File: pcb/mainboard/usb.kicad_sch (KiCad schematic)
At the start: 39 parts

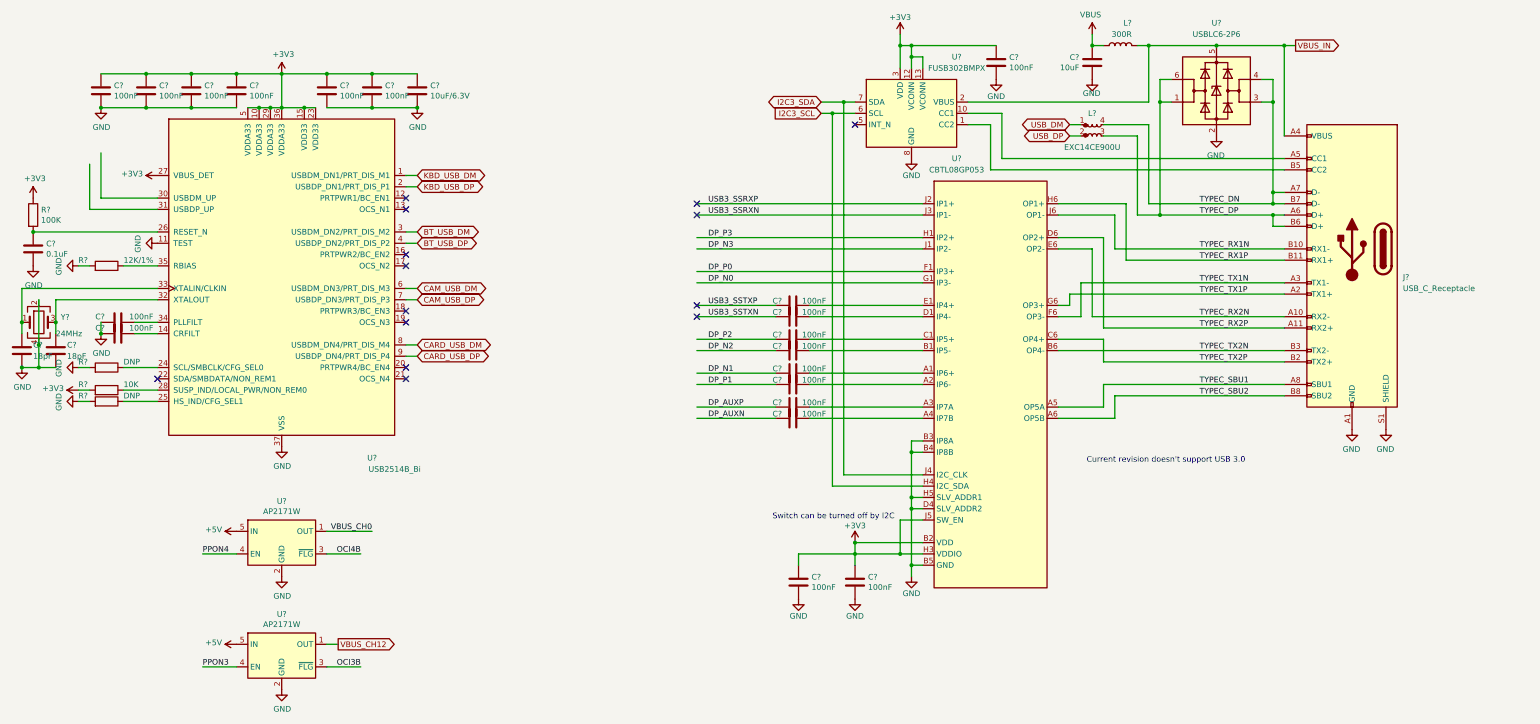
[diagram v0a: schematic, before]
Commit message: - pcb: working on r0p1 sch
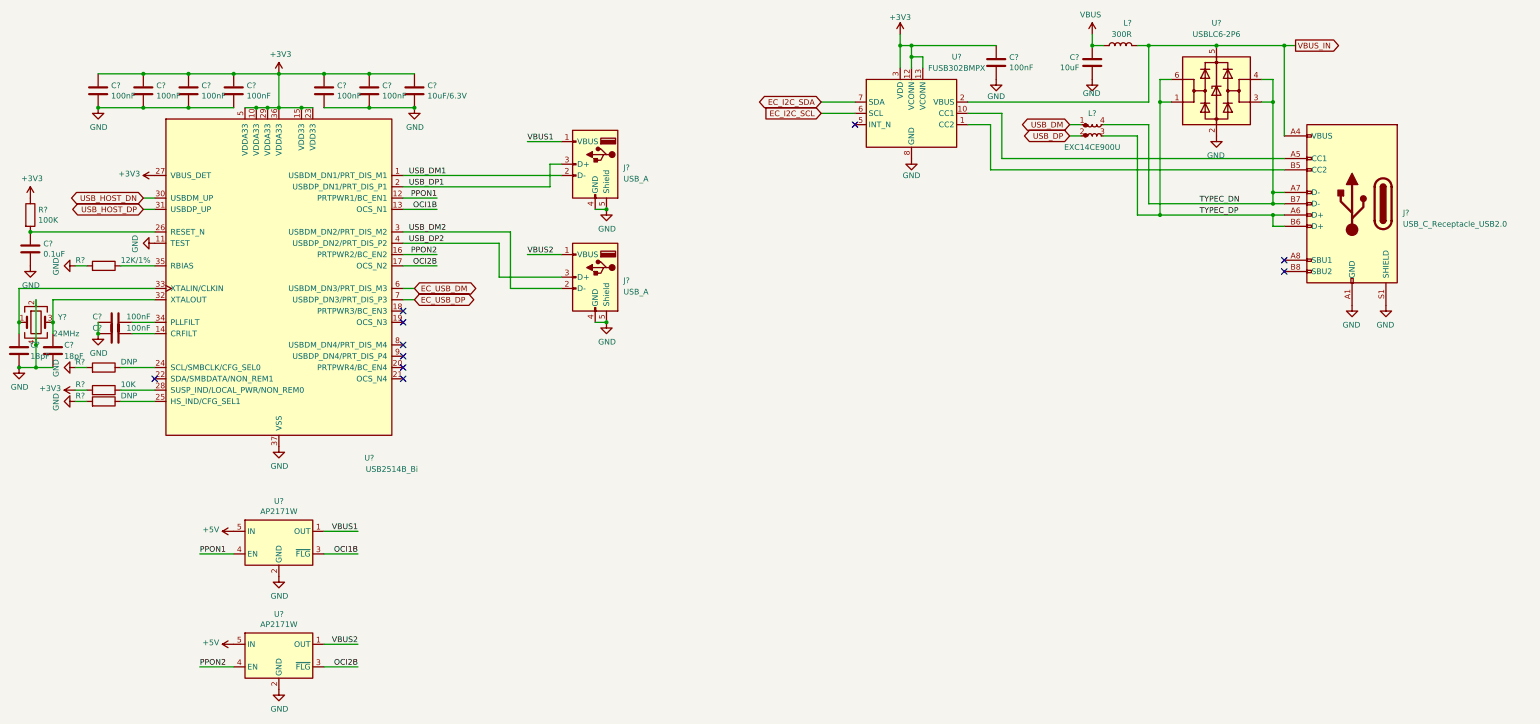
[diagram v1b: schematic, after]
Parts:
- removed C? (x10): 100nF, Capacitor_SMD:C_0201_0603Metric, symbol Device:C
- removed J?: USB_C_Receptacle, Connector_USB:USB_C_Receptacle_Amphenol_12401548E4-2A, symbol Connector:USB_C_Receptacle
- removed U?: CBTL08GP053, footprint:BGA-40_6x9_3.5x5.0mm, symbol symbols:CBTL08GP053
- added J? (x2): USB_A, Connector_USB:USB_A_Molex_67643_Horizontal, symbol Connector:USB_A
- added J?: USB_C_Receptacle_USB2.0, Connector_USB:USB_C_Receptacle_HRO_TYPE-C-31-M-12, symbol Connector:USB_C_Receptacle_USB2.0
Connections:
- net OCI3B is gone; now on net OCI2B: U?.3 (~FLG)
- net OCI4B is gone; now on net OCI1B: U?.3 (~FLG)
- net PPON3 is gone; now on net PPON2: U?.4 (EN)
- net PPON4 is gone; now on net PPON1: U?.4 (EN)
- net GND: now also J?.4 (GND), J?.4 (GND), J?.5 (Shield), J?.5 (Shield), J?.A1 (GND), J?.A12 (GND), J?.B1 (GND), J?.B12 (GND), J?.S1 (SHIELD)
- net TYPEC_DN: now also J?.A7 (D-), J?.B7 (D-)
- net TYPEC_DP: now also J?.A6 (D+), J?.B6 (D+)
- net VBUS_IN: now also J?.A4 (VBUS), J?.A9 (VBUS), J?.B4 (VBUS), J?.B9 (VBUS)
- net PPON1: now reaches U?.12 (PRTPWR1/BC_EN1)
- net OCI1B: now reaches U?.13 (OCS_N1)
- net PPON2: now reaches U?.16 (PRTPWR2/BC_EN2)
- net OCI2B: now reaches U?.17 (OCS_N2)
- net USB_HOST_DN: now reaches U?.30 (USBDM_UP)
- net USB_HOST_DP: now reaches U?.31 (USBDP_UP)
- net at U?.10 (CC1), U?.11 (CC1): now also J?.A5 (CC1)
- net at U?.1 (CC2), U?.14 (CC2): now also J?.B5 (CC2)
- net BT_USB_DM renamed USB_DM2
- net USB_DM2: now also J?.2 (D-)
- net BT_USB_DP renamed USB_DP2
- net USB_DP2: now also J?.3 (D+)
- net CAM_USB_DM renamed EC_USB_DM
- net CAM_USB_DP renamed EC_USB_DP
- net CARD_USB_DM: no longer names the net of U?.8 (USBDM_DN4/PRT_DIS_M4)
- net CARD_USB_DP: no longer names the net of U?.9 (USBDP_DN4/PRT_DIS_P4)
- net I2C3_SCL renamed EC_I2C_SCL
- net I2C3_SDA renamed EC_I2C_SDA
- net KBD_USB_DM renamed USB_DM1
- net USB_DM1: now also J?.2 (D-)
- net KBD_USB_DP renamed USB_DP1
- net USB_DP1: now also J?.3 (D+)
- net VBUS_CH0 renamed VBUS1
- net VBUS1: now also J?.1 (VBUS)
- net VBUS_CH12 renamed VBUS2
- net VBUS2: now also J?.1 (VBUS)
- no-connect marks 14 -> 10
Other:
- note removed: "Current revision doesn't support USB 3.0"
- note removed: "Switch can be turned off by I2C"
- moved on the sheet: C?, R?, U?, Y?
